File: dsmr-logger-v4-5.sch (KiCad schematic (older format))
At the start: 43 parts, among them J1 RJ12 female connector (6P6C), J2 Jack-DC, J3 DC-or-SM-power, J4 I2C conn, J5 Programmer, J6 Test 3v3, J7 Test 5volt, J9 ADC 0-5v, Q1 BC547, SW1 RESET, SW2 FLASH, U1 LM2937xMP, U2 4N35, U3 ESP-12E

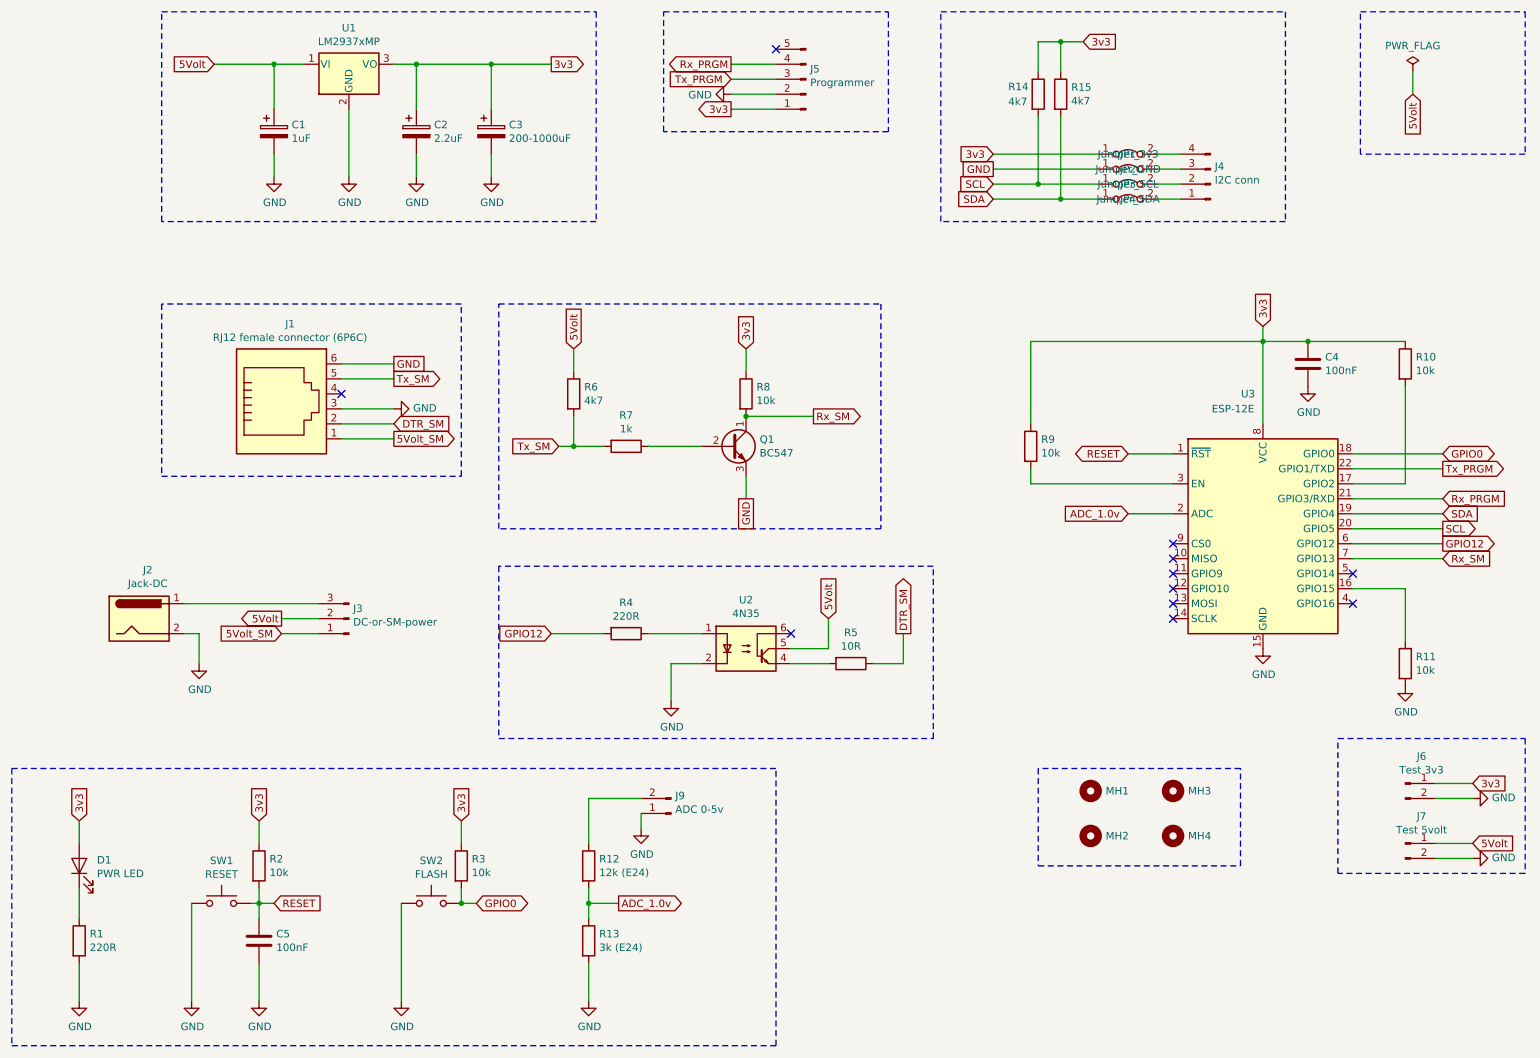
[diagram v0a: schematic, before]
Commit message: Add pcb layout
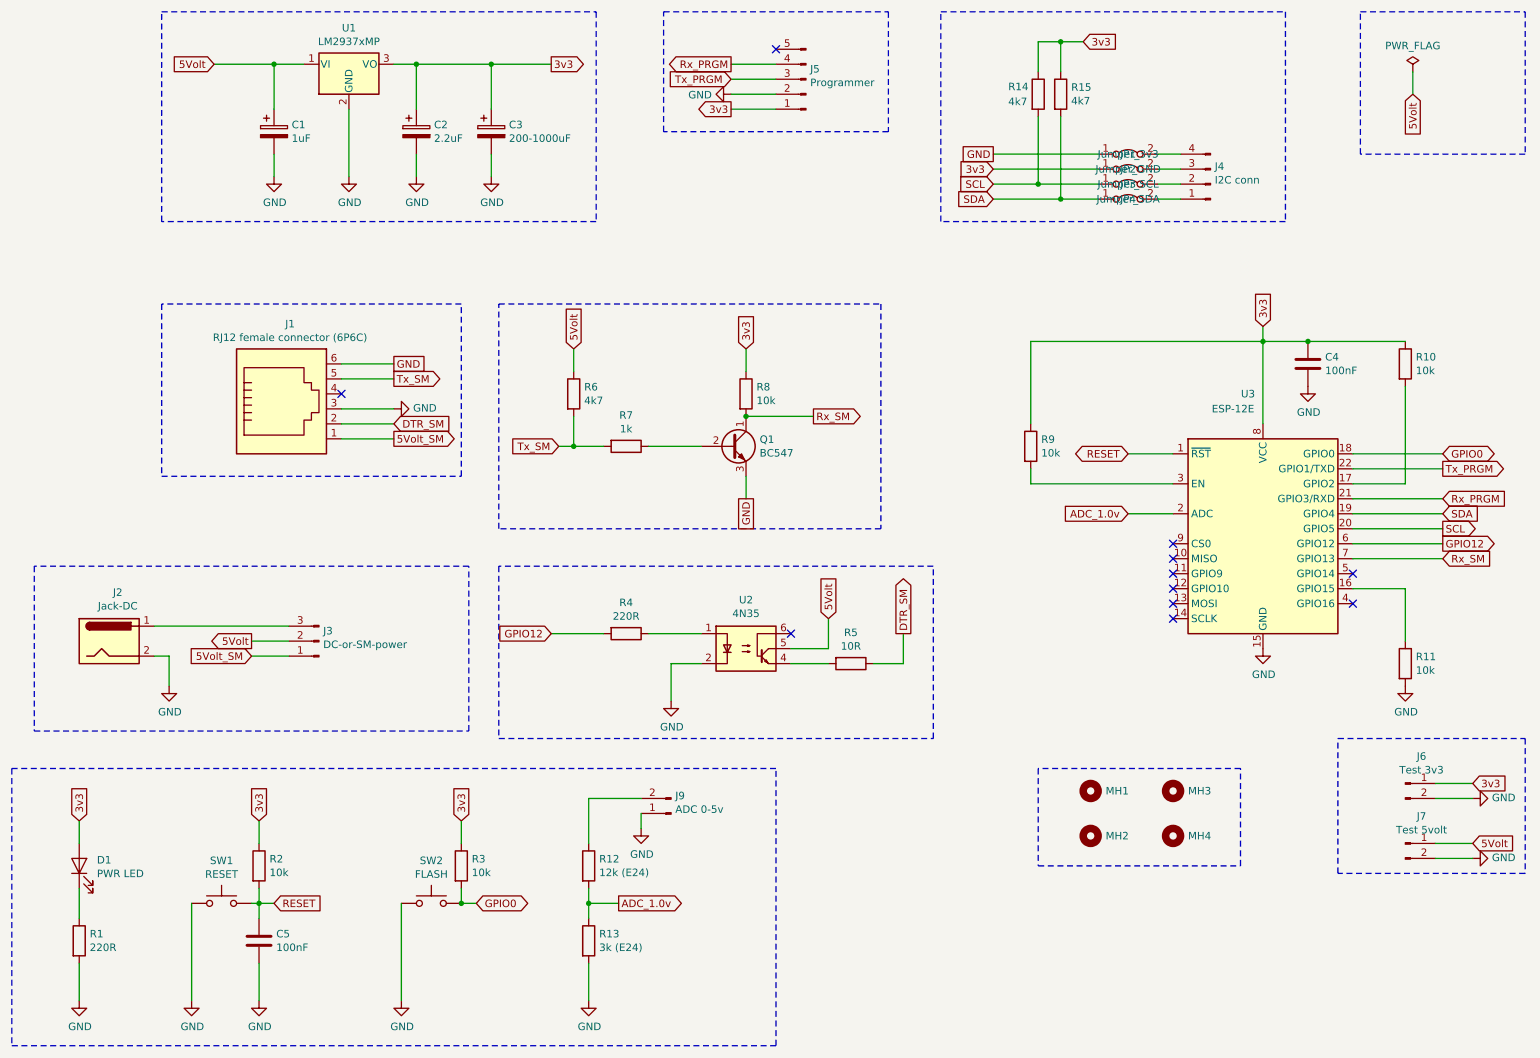
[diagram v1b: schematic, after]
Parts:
- C1: footprint Capacitor_THT:CP_Radial_D5.0mm_P2.50mm -> Capacitor_THT:CP_Radial_D5.0mm_P2.00mm
- C2: footprint Capacitor_THT:CP_Radial_D6.3mm_P2.50mm -> Capacitor_THT:CP_Radial_D5.0mm_P2.00mm
- C3: footprint Capacitor_THT:CP_Radial_D10.0mm_P3.50mm -> Capacitor_THT:CP_Radial_D8.0mm_P5.00mm
- C4, C5: footprint Capacitor_THT:C_Disc_D3.0mm_W1.6mm_P2.50mm -> Capacitor_THT:C_Disc_D5.0mm_W2.5mm_P5.00mm
- D1: footprint LED_THT:LED_D5.0mm -> LED_THT:LED_D3.0mm
- J1: footprint (none) -> Connectors-P1:RJ11-6
- J2: footprint (none) -> Connector_BarrelJack:BarrelJack_CUI_PJ-102AH_Horizontal
- SW1: footprint Button_Switch_THT:SW_PUSH_6mm -> Button_Switch_THT:SW_PUSH_6mm_H7.3mm
- SW2: footprint Button_Switch_THT:SW_PUSH_6mm -> Button_Switch_THT:SW_PUSH_6mm_H13mm
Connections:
- net 3v3: now also JP2.1 (A); no longer JP1.1 (A)
- net GND: now also JP1.1 (A); no longer JP2.1 (A)
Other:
- moved on the sheet: J2, J3
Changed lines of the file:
@@
 F 0 "C1" H 2618 1596 50  0000 L CNN
 F 1 "1uF" H 2618 1505 50  0000 L CNN
-F 2 "Capacitor_THT:CP_Radial_D5.0mm_P2.50mm" H 2538 1400 50  0001 C CNN
+F 2 "Capacitor_THT:CP_Radial_D5.0mm_P2.00mm" H 2538 1400 50  0001 C CNN
 F 3 "~" H 2500 1550 50  0001 C CNN
 	1    2500 1550
@@
 F 0 "C2" H 3568 1596 50  0000 L CNN
 F 1 "2.2uF" H 3568 1505 50  0000 L CNN
-F 2 "Capacitor_THT:CP_Radial_D6.3mm_P2.50mm" H 3488 1400 50  0001 C CNN
+F 2 "Capacitor_THT:CP_Radial_D5.0mm_P2.00mm" H 3488 1400 50  0001 C CNN
 F 3 "~" H 3450 1550 50  0001 C CNN
 	1    3450 1550
@@
 F 0 "C3" H 4068 1596 50  0000 L CNN
 F 1 "200-1000uF" H 4068 1505 50  0000 L CNN
-F 2 "Capacitor_THT:CP_Radial_D10.0mm_P3.50mm" H 3988 1400 50  0001 C CNN
+F 2 "Capacitor_THT:CP_Radial_D8.0mm_P5.00mm" H 3988 1400 50  0001 C CNN
 F 3 "~" H 3950 1550 50  0001 C CNN
 	1    3950 1550
@@
 	1    0    0    -1
 $EndComp
-Text GLabel 7300 1700 0    50   Input ~ 0
+Text GLabel 7300 1700 0    50   UnSpc ~ 0
+GND
+Text GLabel 7300 1800 0    50   Input ~ 0
 3v3
-Text GLabel 7300 1800 0    50   UnSpc ~ 0
-GND
 Text GLabel 7300 1900 0    50   Input ~ 0
 SCL
@@
 F 0 "J1" H 2607 3967 50  0000 C CNN
 F 1 "RJ12 female connector (6P6C)" H 2607 3876 50  0000 C CNN
-F 2 "" V 2550 3425 50  0001 C CNN
+F 2 "Connectors-P1:RJ11-6" V 2550 3425 50  0001 C CNN
 F 3 "~" V 2550 3425 50  0001 C CNN
 	1    2550 3400
@@
 F 0 "C4" H 9515 3146 50  0000 L CNN
 F 1 "100nF" H 9515 3055 50  0000 L CNN
-F 2 "Capacitor_THT:C_Disc_D3.0mm_W1.6mm_P2.50mm" H 9438 2950 50  0001 C CNN
+F 2 "Capacitor_THT:C_Disc_D5.0mm_W2.5mm_P5.00mm" H 9438 2950 50  0001 C CNN
 F 3 "~" H 9400 3100 50  0001 C CNN
 	1    9400 3100
@@
 F 0 "D1" V 1239 6332 50  0000 R CNN
 F 1 "PWR LED" V 1148 6332 50  0000 R CNN
-F 2 "LED_THT:LED_D5.0mm" H 1200 6450 50  0001 C CNN
+F 2 "LED_THT:LED_D3.0mm" H 1200 6450 50  0001 C CNN
 F 3 "~" H 1200 6450 50  0001 C CNN
 	1    1200 6450
@@
 F 0 "C5" H 2515 6996 50  0000 L CNN
 F 1 "100nF" H 2515 6905 50  0000 L CNN
-F 2 "Capacitor_THT:C_Disc_D3.0mm_W1.6mm_P2.50mm" H 2438 6800 50  0001 C CNN
+F 2 "Capacitor_THT:C_Disc_D5.0mm_W2.5mm_P5.00mm" H 2438 6800 50  0001 C CNN
 F 3 "~" H 2400 6950 50  0001 C CNN
 	1    2400 6950
@@
 F 0 "SW1" H 2150 6985 50  0000 C CNN
 F 1 "RESET" H 2150 6894 50  0000 C CNN
-F 2 "Button_Switch_THT:SW_PUSH_6mm" H 2150 6900 50  0001 C CNN
+F 2 "Button_Switch_THT:SW_PUSH_6mm_H7.3mm" H 2150 6900 50  0001 C CNN
 F 3 "~" H 2150 6900 50  0001 C CNN
 	1    2150 6700
@@
 F 0 "SW2" H 3550 6985 50  0000 C CNN
 F 1 "FLASH" H 3550 6894 50  0000 C CNN
-F 2 "Button_Switch_THT:SW_PUSH_6mm" H 3550 6900 50  0001 C CNN
+F 2 "Button_Switch_THT:SW_PUSH_6mm_H13mm" H 3550 6900 50  0001 C CNN
 F 3 "~" H 3550 6900 50  0001 C CNN
 	1    3550 6700
@@
 L Connector:Jack-DC J2
 U 1 1 5E112C34
-P 1600 4800
-F 0 "J2" H 1657 5125 50  0000 C CNN
-F 1 "Jack-DC" H 1657 5034 50  0000 C CNN
-F 2 "" H 1650 4760 50  0001 C CNN
-F 3 "~" H 1650 4760 50  0001 C CNN
-	1    1600 4800
+P 1400 4950
+F 0 "J2" H 1457 5275 50  0000 C CNN
+F 1 "Jack-DC" H 1457 5184 50  0000 C CNN
+F 2 "Connector_BarrelJack:BarrelJack_CUI_PJ-102AH_Horizontal" H 1450 4910 50  0001 C CNN
+F 3 "~" H 1450 4910 50  0001 C CNN
+	1    1400 4950
 	1    0    0    -1
 $EndComp
@@
 L Connector:Conn_01x03_Male J3
 U 1 1 5E113AD6
-P 3000 4800
-F 0 "J3" H 2972 4732 50  0000 R CNN
-F 1 "DC-or-SM-power" H 2972 4823 50  0000 R CNN
-F 2 "Connector_PinHeader_2.54mm:PinHeader_1x03_P2.54mm_Vertical" H 3000 4800 50  0001 C CNN
-F 3 "~" H 3000 4800 50  0001 C CNN
-	1    3000 4800
+P 2800 4950
+F 0 "J3" H 2772 4882 50  0000 R CNN
+F 1 "DC-or-SM-power" H 2772 4973 50  0000 R CNN
+F 2 "Connector_PinHeader_2.54mm:PinHeader_1x03_P2.54mm_Vertical" H 2800 4950 50  0001 C CNN
+F 3 "~" H 2800 4950 50  0001 C CNN
+	1    2800 4950
 	-1   0    0    1
 $EndComp
@@
 L power:GND #PWR0114
 U 1 1 5E118460
-P 2000 5100
-F 0 "#PWR0114" H 2000 4850 50  0001 C CNN
-F 1 "GND" H 2005 4927 50  0000 C CNN
-F 2 "" H 2000 5100 50  0001 C CNN
-F 3 "" H 2000 5100 50  0001 C CNN
-	1    2000 5100
-	1    0    0    -1
-$EndComp
-Text GLabel 2550 4900 0    50   Input ~ 0
+P 1800 5250
+F 0 "#PWR0114" H 1800 5000 50  0001 C CNN
+F 1 "GND" H 1805 5077 50  0000 C CNN
+F 2 "" H 1800 5250 50  0001 C CNN
+F 3 "" H 1800 5250 50  0001 C CNN
+	1    1800 5250
+	1    0    0    -1
+$EndComp
+Text GLabel 2350 5050 0    50   Input ~ 0
 5Volt_SM
 Wire Wire Line
-	2550 4900 2800 4900
-Wire Wire Line
-	1900 4700 2800 4700
-Text GLabel 2550 4800 0    50   Output ~ 0
+	2350 5050 2600 5050
+Wire Wire Line
+	1700 4850 2600 4850
+Text GLabel 2350 4950 0    50   Output ~ 0
 5Volt
 $Comp
@@
 $EndComp
 Wire Wire Line
-	1900 4900 2000 4900
-Wire Wire Line
-	2000 4900 2000 5100
-Wire Wire Line
-	2550 4800 2800 4800
+	1700 5050 1800 5050
+Wire Wire Line
+	1800 5050 1800 5250
+Wire Wire Line
+	2350 4950 2600 4950
+Wire Notes Line
+	3800 4450 900  4450
+Wire Notes Line
+	900  4450 900  5550
+Wire Notes Line
+	900  5550 3800 5550
+Wire Notes Line
+	3800 5550 3800 4450
 $EndSCHEMATC
